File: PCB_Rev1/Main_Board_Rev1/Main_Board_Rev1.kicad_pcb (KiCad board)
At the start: 4 copper layers, 152.4 x 152.4 mm, 84 parts, among them IC1 LT8648SEV#PBF, J1 PRT-14017, J10 B4B-PH-K-S, J11 532610771, J12 532610771, J13 532610771, J2 Conn_01x04_Socket, J3 691137710002, J4 Conn_01x02_Pin, J5 XT60PW-M, J6 Conn_01x02_Pin, J7 Conn_01x02_Pin, J8 Conn_01x02_Pin, J9 B4B-PH-K-S, Q1 AO3400A, Q2 AO3400A, Q3 AO3400A, Q4 IRFHM9331TRPBF, U1 AZ1117IH-3.3TRG1, U2 L298N, X1 B2P-VH, X2 B2P-VH

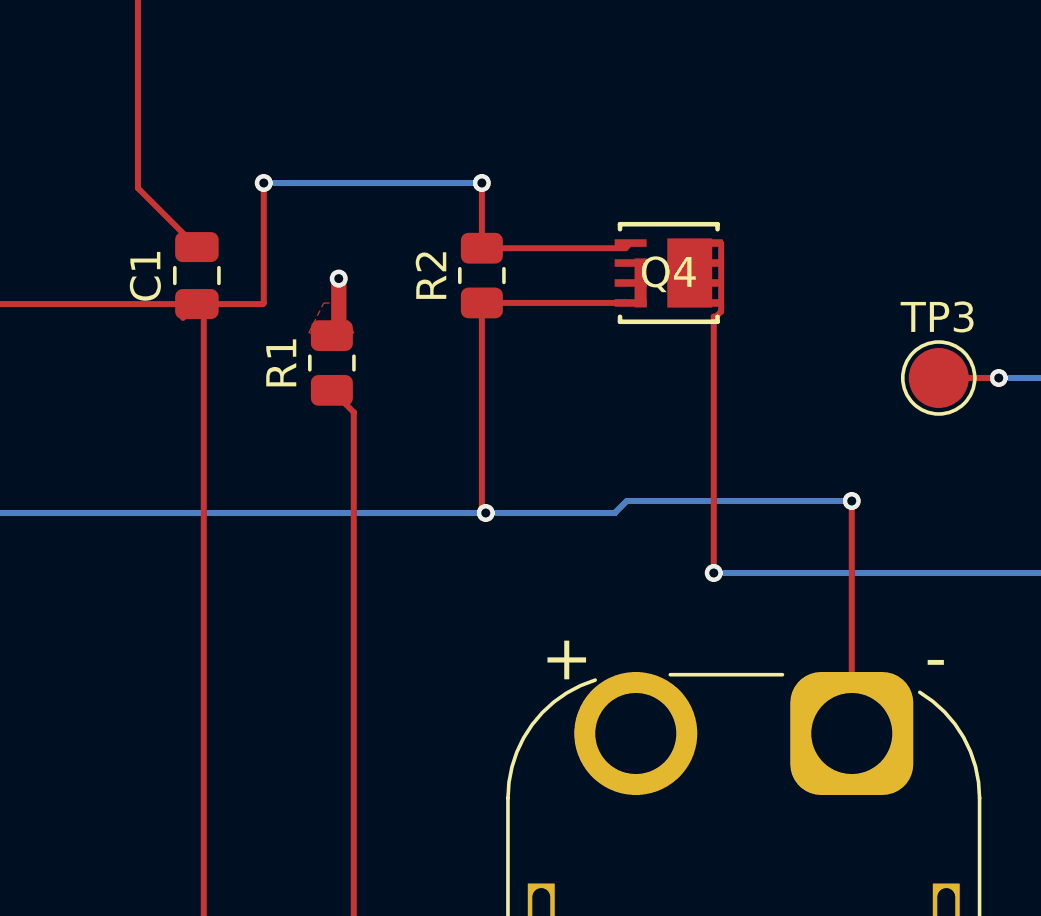
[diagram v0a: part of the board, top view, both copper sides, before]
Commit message: Routing
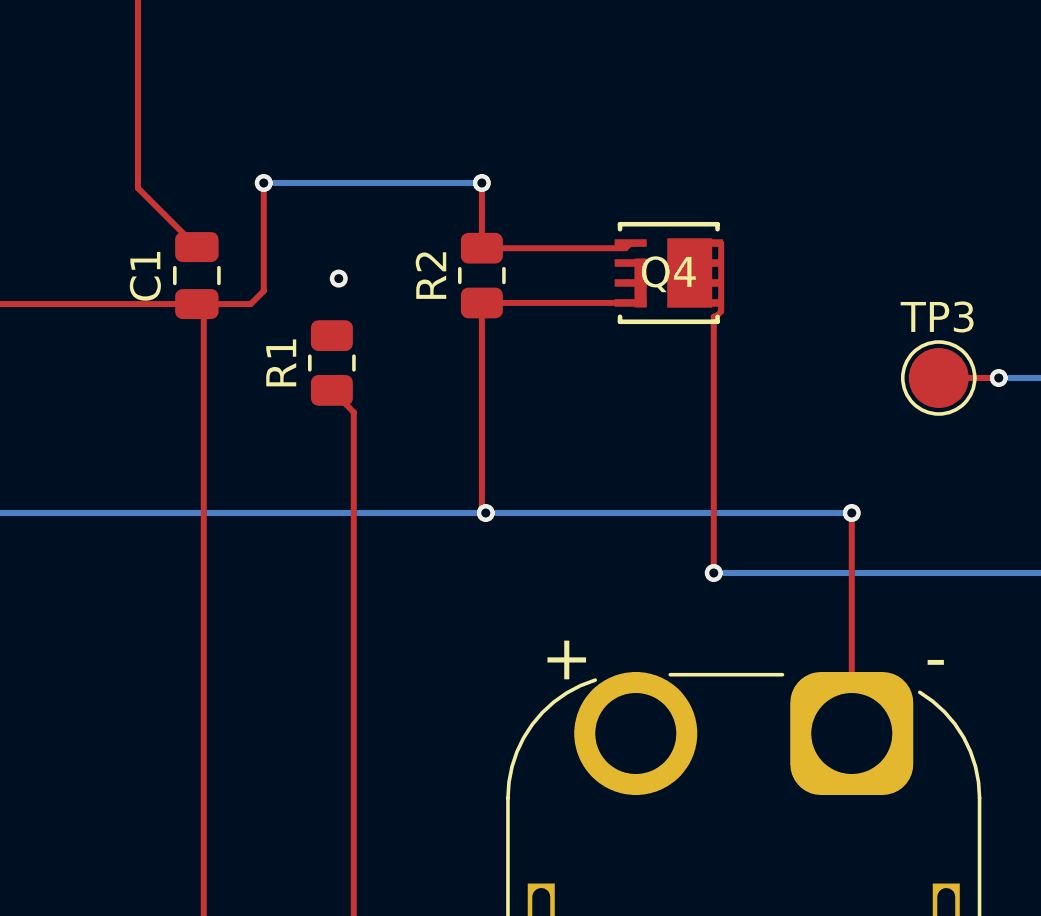
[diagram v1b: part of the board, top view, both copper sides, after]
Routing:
- net GND: track 360.0 -> 358.4 mm
- net Net-(C1-Pad1): track 61.2 -> 60.3 mm
- net BATT_IN: track 53.5 -> 52.8 mm
- removed copper zone on F.Cu, net GND
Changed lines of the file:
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@@
 	)
 	(segment
-		(start 40 140)
-		(end 39.96428 140.03572)
+		(start 47.27 138.17322)
+		(end 52.05856 138.17322)
 		(width 0.2)
 		(layer "F.Cu")
@@
 	)
 	(segment
-		(start 47.27 138.17322)
-		(end 52.05856 138.17322)
+		(start 26.43572 140.03572)
+		(end 37.77 140.03572)
 		(width 0.2)
 		(layer "F.Cu")
@@
 	)
 	(segment
-		(start 26.43572 140.03572)
+		(start 39.56428 140.03572)
 		(end 37.77 140.03572)
 		(width 0.2)
@@
 	)
 	(segment
-		(start 37.3075 140.49822)
-		(end 37.77 140.03572)
-		(width 0.2)
-		(layer "F.Cu")
-		(net 1)
-	)
-	(segment
 		(start 25.8 139.6)
 		(end 26 139.6)
@@
 	)
 	(segment
-		(start 40 136)
-		(end 40 140)
+		(start 38 140.26572)
+		(end 37.77 140.03572)
 		(width 0.2)
 		(layer "F.Cu")
@@
 	)
 	(segment
-		(start 38 140.26572)
-		(end 37.77 140.03572)
+		(start 40 139.6)
+		(end 39.56428 140.03572)
 		(width 0.2)
 		(layer "F.Cu")
@@
 	)
 	(segment
-		(start 38 167.5)
-		(end 38 140.26572)
+		(start 40 136)
+		(end 40 139.6)
 		(width 0.2)
 		(layer "F.Cu")
@@
 	)
 	(segment
-		(start 39.96428 140.03572)
-		(end 37.77 140.03572)
+		(start 38 167.5)
+		(end 38 140.26572)
 		(width 0.2)
 		(layer "F.Cu")
@@
 	)
 	(segment
-		(start 42.5 140.81375)
-		(end 42.5 139.18625)
-		(width 0.508)
-		(layer "F.Cu")
-		(net 2)
-	)
-	(segment
 		(start 35.8055 136.17122)
 		(end 37.77 138.13572)
@@
 	)
 	(segment
-		(start 59.6 154.35)
-		(end 59.6 146.6)
-		(width 0.2)
-		(layer "F.Cu")
-		(net 36)
-	)
-	(segment
 		(start 47.4 147)
 		(end 47.27 146.87)
@@
 	)
 	(segment
-		(start 59.5 146.5)
-		(end 59.6 146.6)
+		(start 30.2 147)
+		(end 26 147)
 		(width 0.2)
 		(layer "F.Cu")
@@
 	)
 	(segment
-		(start 30.2 147)
-		(end 26 147)
+		(start 59.6 154.35)
+		(end 59.6 147)
 		(width 0.2)
 		(layer "F.Cu")
@@
 	)
 	(via
-		(at 59.6 146.6)
+		(at 59.6 147)
 		(size 0.6)
 		(drill 0.3)
@@
 	)
 	(segment
-		(start 59.6 146.6)
-		(end 52.1 146.6)
-		(width 0.2)
-		(layer "B.Cu")
-		(net 36)
-	)
-	(segment
-		(start 52.1 146.6)
-		(end 51.7 147)
-		(width 0.2)
-		(layer "B.Cu")
-		(net 36)
-	)
-	(segment
-		(start 51.7 147)
+		(start 59.6 147)
 		(end 47.4 147)
 		(width 0.2)
@@
 	)
 	(zone
-		(net 2)
-		(net_name "GND")
-		(layer "F.Cu")
-		(hatch full 0.5)
-		(priority 1)
-		(connect_pads yes
-			(clearance 0.5)
-		)
-		(min_thickness 0.25)
-		(filled_areas_thickness no)
-		(fill yes
-			(thermal_gap 0.5)
-			(thermal_bridge_width 0.5)
-		)
-		(polygon
-			(pts
-				(xy 42 140) (xy 42.5 140) (xy 43 141) (xy 41.5 141)
-			)
-		)
-	)
-	(zone
